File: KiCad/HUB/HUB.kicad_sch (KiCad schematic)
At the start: 2 parts, among them J1 ESP8266(wifi)

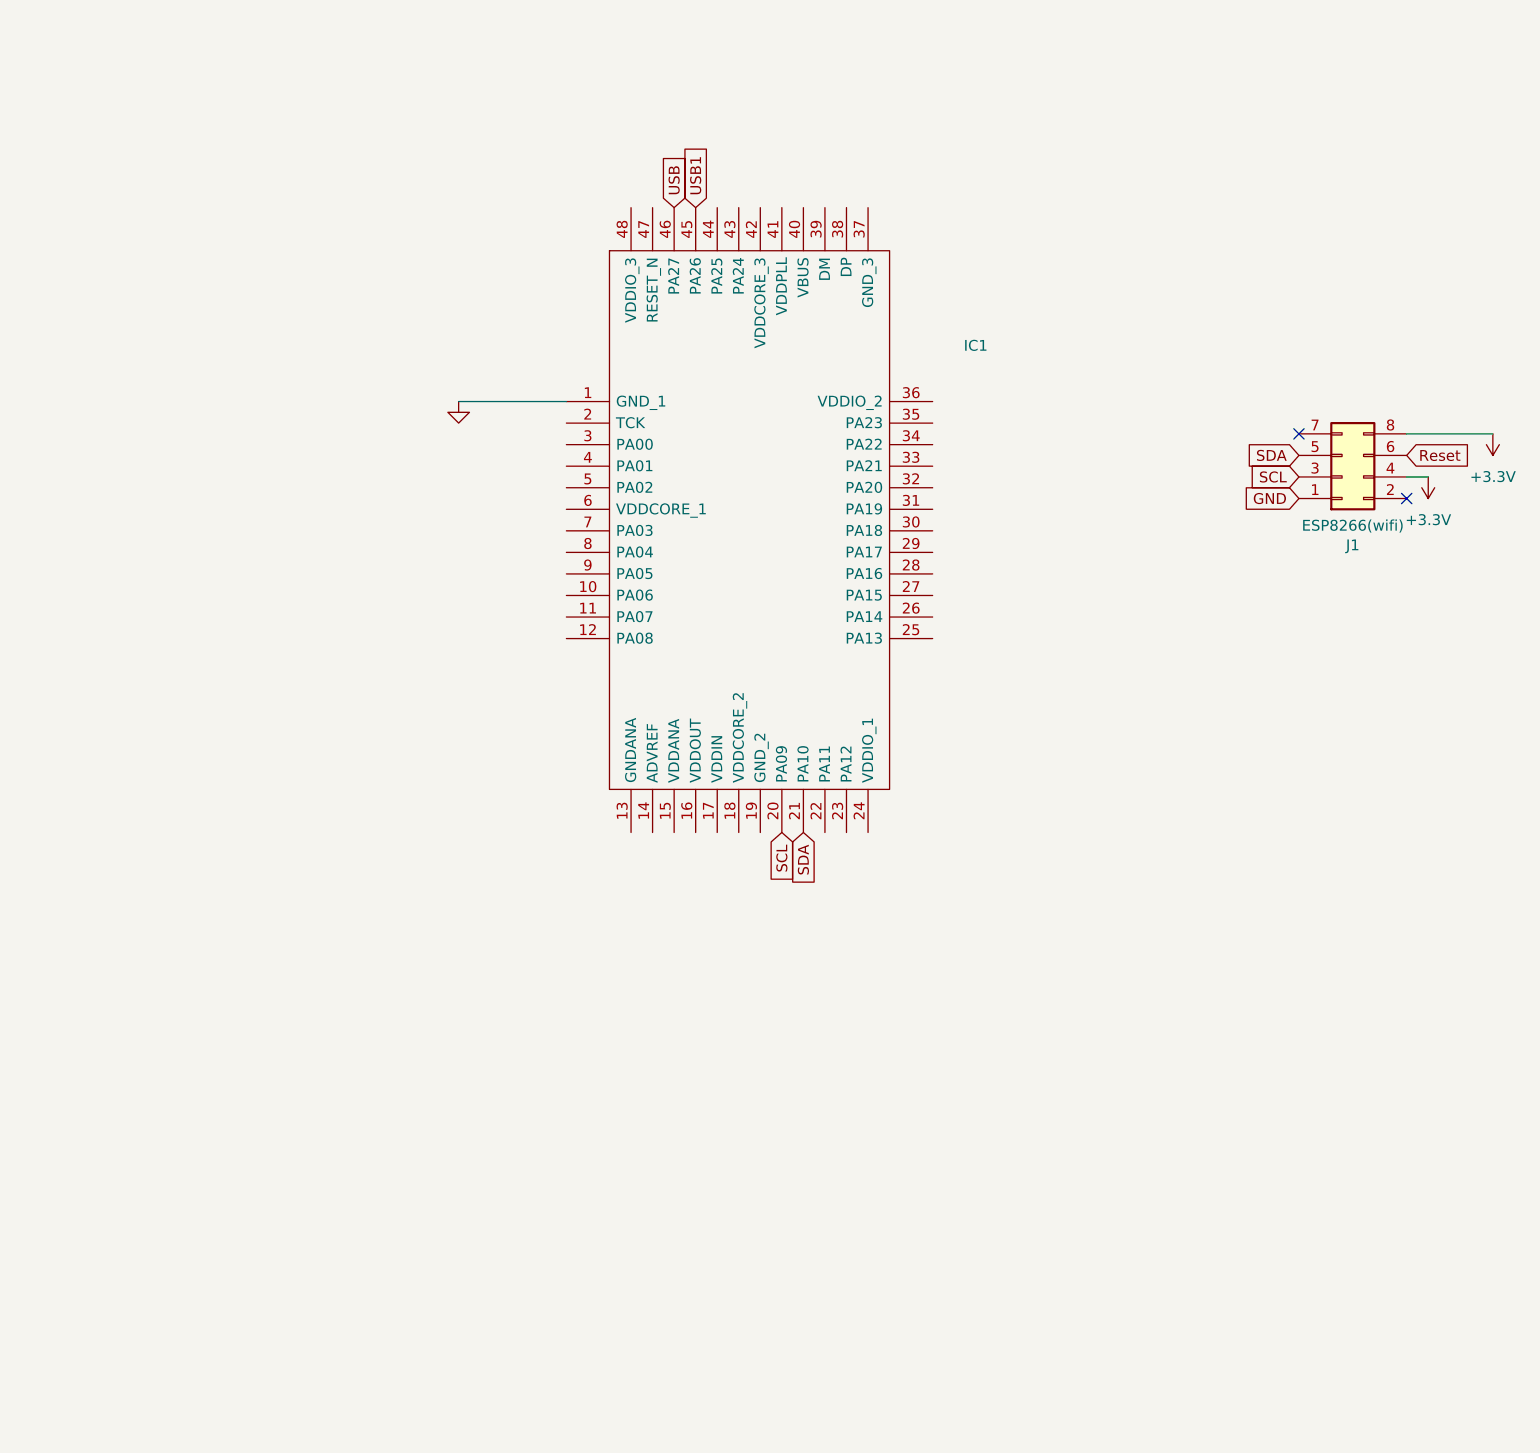
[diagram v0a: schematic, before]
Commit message: hub
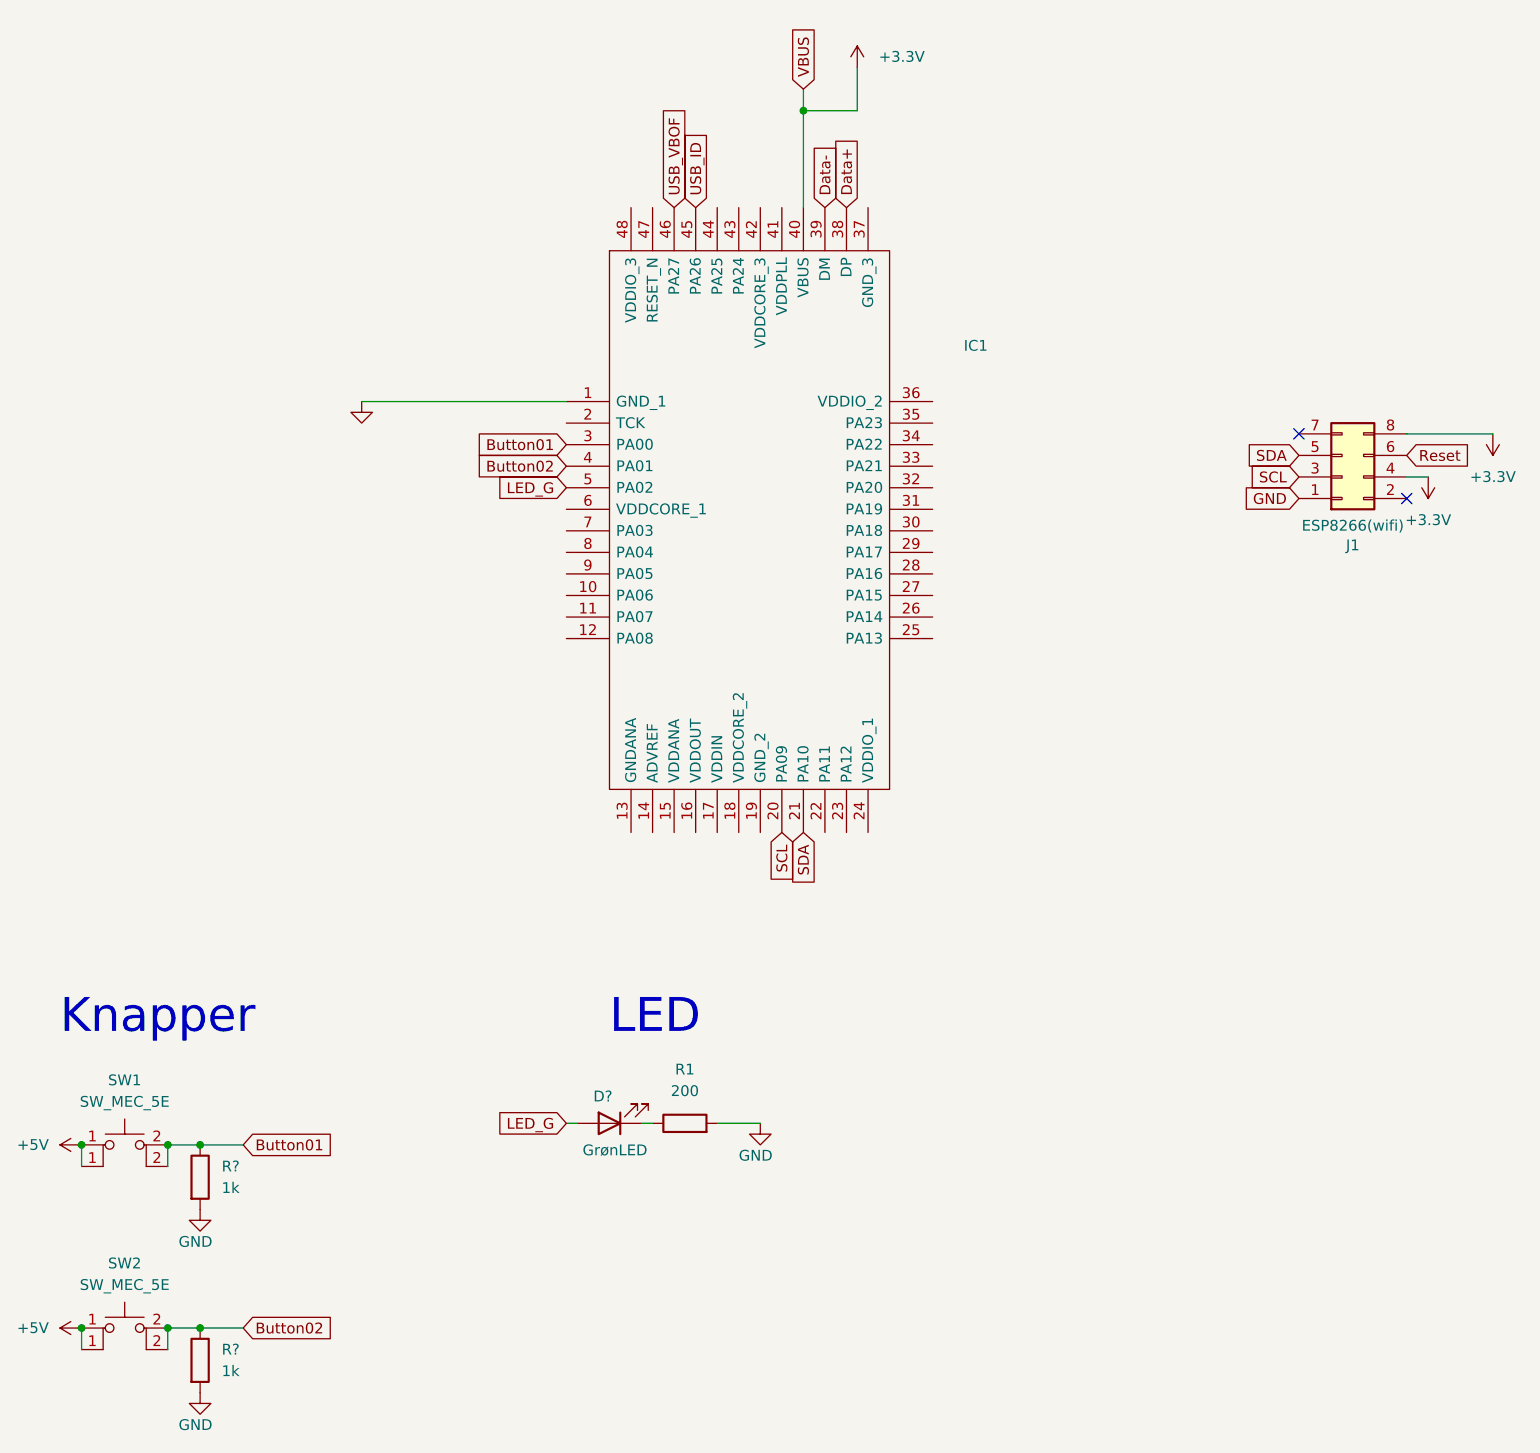
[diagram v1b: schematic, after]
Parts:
- added D?: GrønLED, LED_THT:LED_D3.0mm_FlatTop, symbol Device:LED
- added R1: 200, Resistor_THT:R_Axial_DIN0309_L9.0mm_D3.2mm_P12.70mm_Horizontal, symbol Device:R
- added R? (x2): 1k, Resistor_THT:R_Axial_DIN0309_L9.0mm_D3.2mm_P12.70mm_Horizontal, symbol Device:R
- added SW1, SW2: SW_MEC_5E, Button_Switch_THT:SW_PUSH_6mm_H4.3mm, symbol Switch:SW_MEC_5E
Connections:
- net +3V3: now also IC1.40 (VBUS)
- net GND: now also R1.2, R?.2, R?.2
- net Button01: now reaches IC1.3 (PA00)
- net Button01: now also R?.1, SW1.2 (K)
- net Data+: now reaches IC1.38 (DP)
- net Data-: now reaches IC1.39 (DM)
- net Button02: now reaches IC1.4 (PA01)
- net Button02: now also R?.1, SW2.2 (K)
- net LED_G: now reaches IC1.5 (PA02)
- net LED_G: now also D?.2 (A)
- net USB renamed USB_VBOF
- net USB1 renamed USB_ID
- new net: D?.1 (K), R1.1
- new net +5V: SW1.1 (2), SW2.1 (2)
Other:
- note added: "Knapper"
- note added: "LED"
